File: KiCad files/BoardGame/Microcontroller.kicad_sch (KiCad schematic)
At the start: 11 parts, among them J501 USBasp, SW501 SW_Push, U501 ATmega328P-A, Y501 16MHz

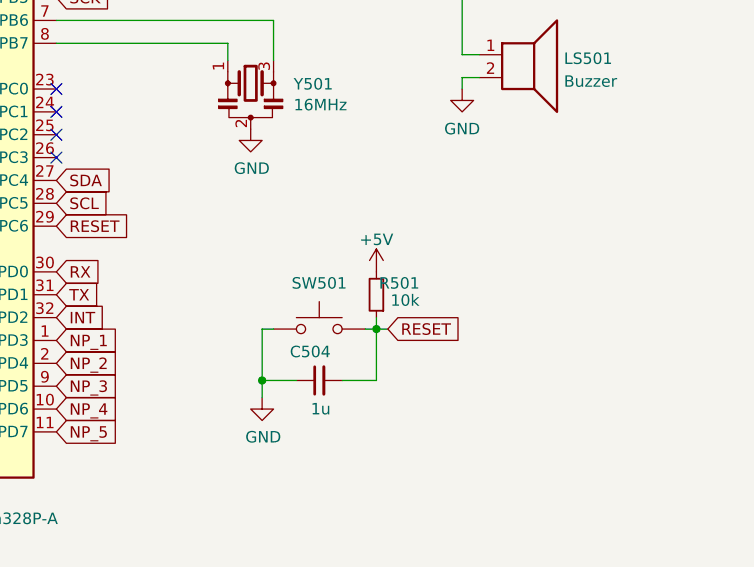
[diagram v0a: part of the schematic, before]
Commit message: update
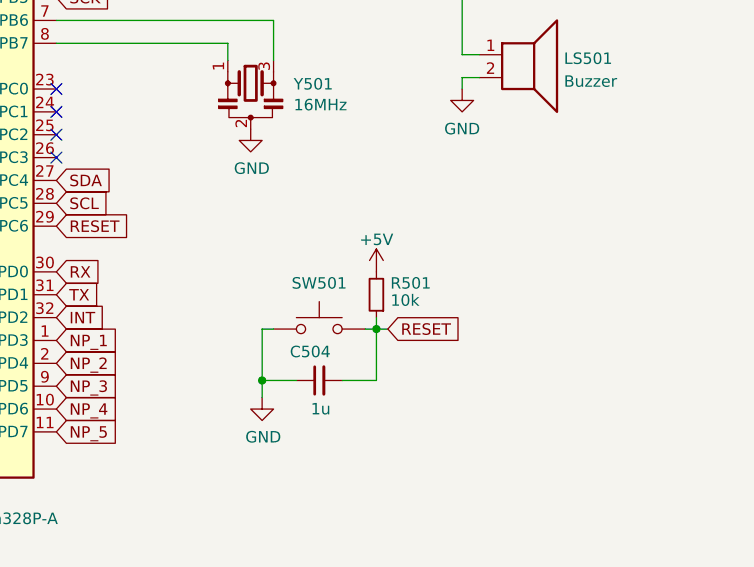
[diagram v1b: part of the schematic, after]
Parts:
- C501, C502, C503: JLCPCB Part # (none) -> C113803; U labosu? (none) -> ne
- C504: JLCPCB Part # (none) -> C559769; U labosu? (none) -> da
- J501: JLCPCB Part # (none) -> -; Ostalo (none) -> -; U labosu? (none) -> da
- L501: JLCPCB Part # (none) -> C281117; U labosu? (none) -> da
- LS501, R501, U501: U labosu? (none) -> da
- SW501: JLCPCB Part # (none) -> C2886894; U labosu? (none) -> ne
- Y501: JLCPCB Part # (none) -> C32180; U labosu? (none) -> da
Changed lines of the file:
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@@
+      (effects (font (size 1.27 1.27)) hide)
+    )
+    (property "JLCPCB Part #" "C2886894" (id 4) (at 177.165 125.095 0)
+      (effects (font (size 1.27 1.27)) hide)
+    )
+    (property "U labosu?" "ne" (id 5) (at 177.165 125.095 0)
       (effects (font (size 1.27 1.27)) hide)
     )
@@
   (symbol (lib_id "Device:R_Small") (at 183.515 121.285 180) (unit 1)
     (in_bom yes) (on_board yes)
-    (property "Reference" "R501" (id 0) (at 186.055 120.015 0))
+    (property "Reference" "R501" (id 0) (at 187.325 120.015 0))
     (property "Value" "10k" (id 1) (at 186.69 121.92 0))
     (property "Footprint" "Resistor_SMD:R_0603_1608Metric" (id 2) (at 183.515 121.285 0)
@@
       (effects (font (size 1.27 1.27)) hide)
     )
+    (property "U labosu?" "da" (id 4) (at 183.515 121.285 0)
+      (effects (font (size 1.27 1.27)) hide)
+    )
     (pin "1")
     (pin "2")
@@
       (effects (font (size 1.27 1.27)) hide)
     )
+    (property "U labosu?" "da" (id 4) (at 200.025 94.615 0)
+      (effects (font (size 1.27 1.27)) hide)
+    )
     (pin "1")
     (pin "2")
@@
     )
     (property "Datasheet" "http://ww1.microchip.com/downloads/en/DeviceDoc/ATmega328_P%20AVR%20MCU%20with%20picoPower%20Technology%20Data%20Sheet%2040001984A.pdf" (id 3) (at 132.715 106.045 0)
+      (effects (font (size 1.27 1.27)) hide)
+    )
+    (property "U labosu?" "da" (id 4) (at 132.715 106.045 0)
       (effects (font (size 1.27 1.27)) hide)
     )
@@
       (effects (font (size 1.27 1.27)) hide)
     )
+    (property "U labosu?" "ne" (id 4) (at 90.805 66.04 0)
+      (effects (font (size 1.27 1.27)) hide)
+    )
+    (property "JLCPCB Part #" "C113803" (id 5) (at 90.805 66.04 0)
+      (effects (font (size 1.27 1.27)) hide)
+    )
     (pin "1")
     (pin "2")
@@
       (effects (font (size 1.27 1.27)) hide)
     )
+    (property "U labosu?" "ne" (id 4) (at 154.305 67.31 0)
+      (effects (font (size 1.27 1.27)) hide)
+    )
+    (property "JLCPCB Part #" "C113803" (id 5) (at 154.305 67.31 0)
+      (effects (font (size 1.27 1.27)) hide)
+    )
     (pin "1")
     (pin "2")
@@
       (effects (font (size 1.27 1.27)) hide)
     )
+    (property "JLCPCB Part #" "C32180" (id 4) (at 169.545 97.79 0)
+      (effects (font (size 1.27 1.27)) hide)
+    )
+    (property "U labosu?" "da" (id 5) (at 169.545 97.79 0)
+      (effects (font (size 1.27 1.27)) hide)
+    )
     (pin "1")
     (pin "2")
@@
       (effects (font (size 1.27 1.27)) hide)
     )
+    (property "JLCPCB Part #" "C559769" (id 4) (at 177.165 130.81 0)
+      (effects (font (size 1.27 1.27)) hide)
+    )
+    (property "U labosu?" "da" (id 5) (at 177.165 130.81 0)
+      (effects (font (size 1.27 1.27)) hide)
+    )
     (pin "1")
     (pin "2")
@@
       (effects (font (size 1.27 1.27)) hide)
     )
+    (property "JLCPCB Part #" "C281117" (id 4) (at 154.305 56.515 0)
+      (effects (font (size 1.27 1.27)) hide)
+    )
+    (property "U labosu?" "da" (id 5) (at 154.305 56.515 0)
+      (effects (font (size 1.27 1.27)) hide)
+    )
     (pin "1")
     (pin "2")
@@
     )
     (property "Datasheet" "~" (id 3) (at 105.41 82.55 0)
+      (effects (font (size 1.27 1.27)) hide)
+    )
+    (property "U labosu?" "ne" (id 4) (at 105.41 82.55 0)
+      (effects (font (size 1.27 1.27)) hide)
+    )
+    (property "JLCPCB Part #" "C113803" (id 5) (at 105.41 82.55 0)
       (effects (font (size 1.27 1.27)) hide)
     )
@@
       (effects (font (size 1.27 1.27)) hide)
     )
+    (property "JLCPCB Part #" "-" (id 4) (at 207.01 63.5 0)
+      (effects (font (size 1.27 1.27)) hide)
+    )
+    (property "Ostalo" "-" (id 5) (at 207.01 63.5 0)
+      (effects (font (size 1.27 1.27)) hide)
+    )
+    (property "U labosu?" "da" (id 6) (at 207.01 63.5 0)
+      (effects (font (size 1.27 1.27)) hide)
+    )

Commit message: update
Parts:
- J501: footprint Footprints:2x03_P2.54mm -> Connector_PinHeader_1.27mm:PinHeader_2x03_P1.27mm_Vertical_SMD
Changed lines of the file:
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@@
     (property "Reference" "J501" (id 0) (at 208.28 58.42 0))
     (property "Value" "USBasp" (id 1) (at 208.28 68.58 0))
-    (property "Footprint" "Footprints:2x03_P2.54mm" (id 2) (at 207.01 63.5 0)
+    (property "Footprint" "Connector_PinHeader_1.27mm:PinHeader_2x03_P1.27mm_Vertical_SMD" (id 2) (at 207.01 63.5 0)
       (effects (font (size 1.27 1.27)) hide)
     )

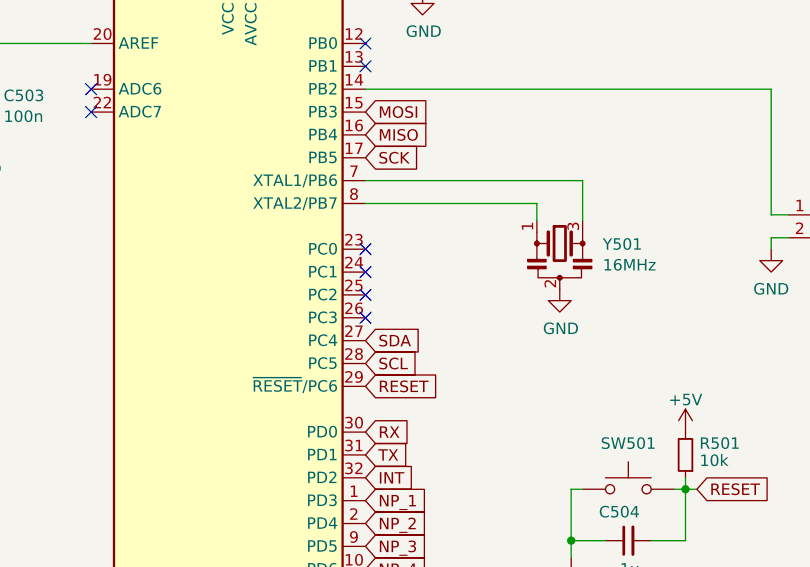
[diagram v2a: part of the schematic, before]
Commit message: update
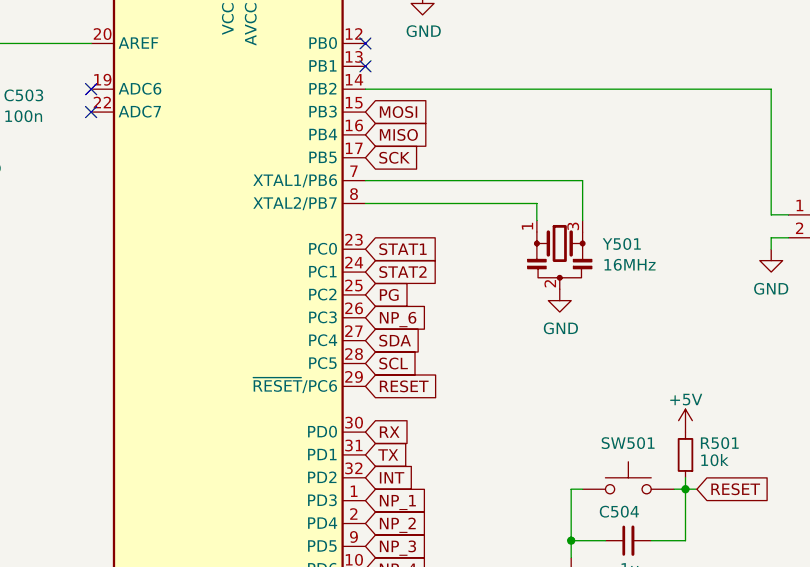
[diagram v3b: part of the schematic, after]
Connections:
- net STAT1: now reaches U501.23 (PC0)
- net STAT2: now reaches U501.24 (PC1)
- net PG: now reaches U501.25 (PC2)
- net NP_6: now reaches U501.26 (PC3)
- no-connect marks 9 -> 5
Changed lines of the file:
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@@
   )
   (no_connect (at 117.475 80.645))
-  (no_connect (at 147.955 100.965))
   (no_connect (at 117.475 83.185))
-  (no_connect (at 147.955 103.505))
   (no_connect (at 214.63 60.96))
-  (no_connect (at 147.955 98.425))
   (no_connect (at 147.955 78.105))
-  (no_connect (at 147.955 106.045))
   (no_connect (at 147.955 75.565))
   (wire (pts (xy 193.04 80.645) (xy 193.04 94.615))
@@
     (effects (font (size 1.27 1.27)) (justify left bottom))
   )
+  (global_label "STAT1" (shape input) (at 147.955 98.425 0) (fields_autoplaced)
+    (effects (font (size 1.27 1.27)) (justify left))
+    (property "Intersheet References" "${INTERSHEET_REFS}" (id 0) (at 155.811 98.3456 0)
+      (effects (font (size 1.27 1.27)) (justify left) hide)
+    )
+  )
   (global_label "MOSI" (shape input) (at 147.955 83.185 0) (fields_autoplaced)
     (effects (font (size 1.27 1.27)) (justify left))
@@
     )
   )
+  (global_label "PG" (shape input) (at 147.955 103.505 0) (fields_autoplaced)
+    (effects (font (size 1.27 1.27)) (justify left))
+    (property "Intersheet References" "${INTERSHEET_REFS}" (id 0) (at 152.9081 103.4256 0)
+      (effects (font (size 1.27 1.27)) (justify left) hide)
+    )
+  )
   (global_label "NP_1" (shape input) (at 147.955 126.365 0) (fields_autoplaced)
     (effects (font (size 1.27 1.27)) (justify left))
@@
     )
   )
+  (global_label "NP_6" (shape input) (at 147.955 106.045 0) (fields_autoplaced)
+    (effects (font (size 1.27 1.27)) (justify left))
+    (property "Intersheet References" "${INTERSHEET_REFS}" (id 0) (at 155.1457 105.9656 0)
+      (effects (font (size 1.27 1.27)) (justify left) hide)
+    )
+  )
   (global_label "NP_2" (shape input) (at 147.955 128.905 0) (fields_autoplaced)
     (effects (font (size 1.27 1.27)) (justify left))
@@
       (effects (font (size 1.27 1.27)) (justify left) hide)
     )
+  )
+  (global_label "STAT2" (shape input) (at 147.955 100.965 0) (fields_autoplaced)
+    (effects (font (size 1.27 1.27)) (justify left))
+    (property "Intersheet References" "${INTERSHEET_REFS}" (id 0) (at 155.811 100.8856 0)
+      (effects (font (size 1.27 1.27)) (justify left) hide)
+    )
